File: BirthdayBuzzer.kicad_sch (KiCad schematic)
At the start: 14 parts, among them J3 Conn_ARM_SWD_TagConnect_TC203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, SW1 SW_Push, U1 PIC18F15Q41-I/SS

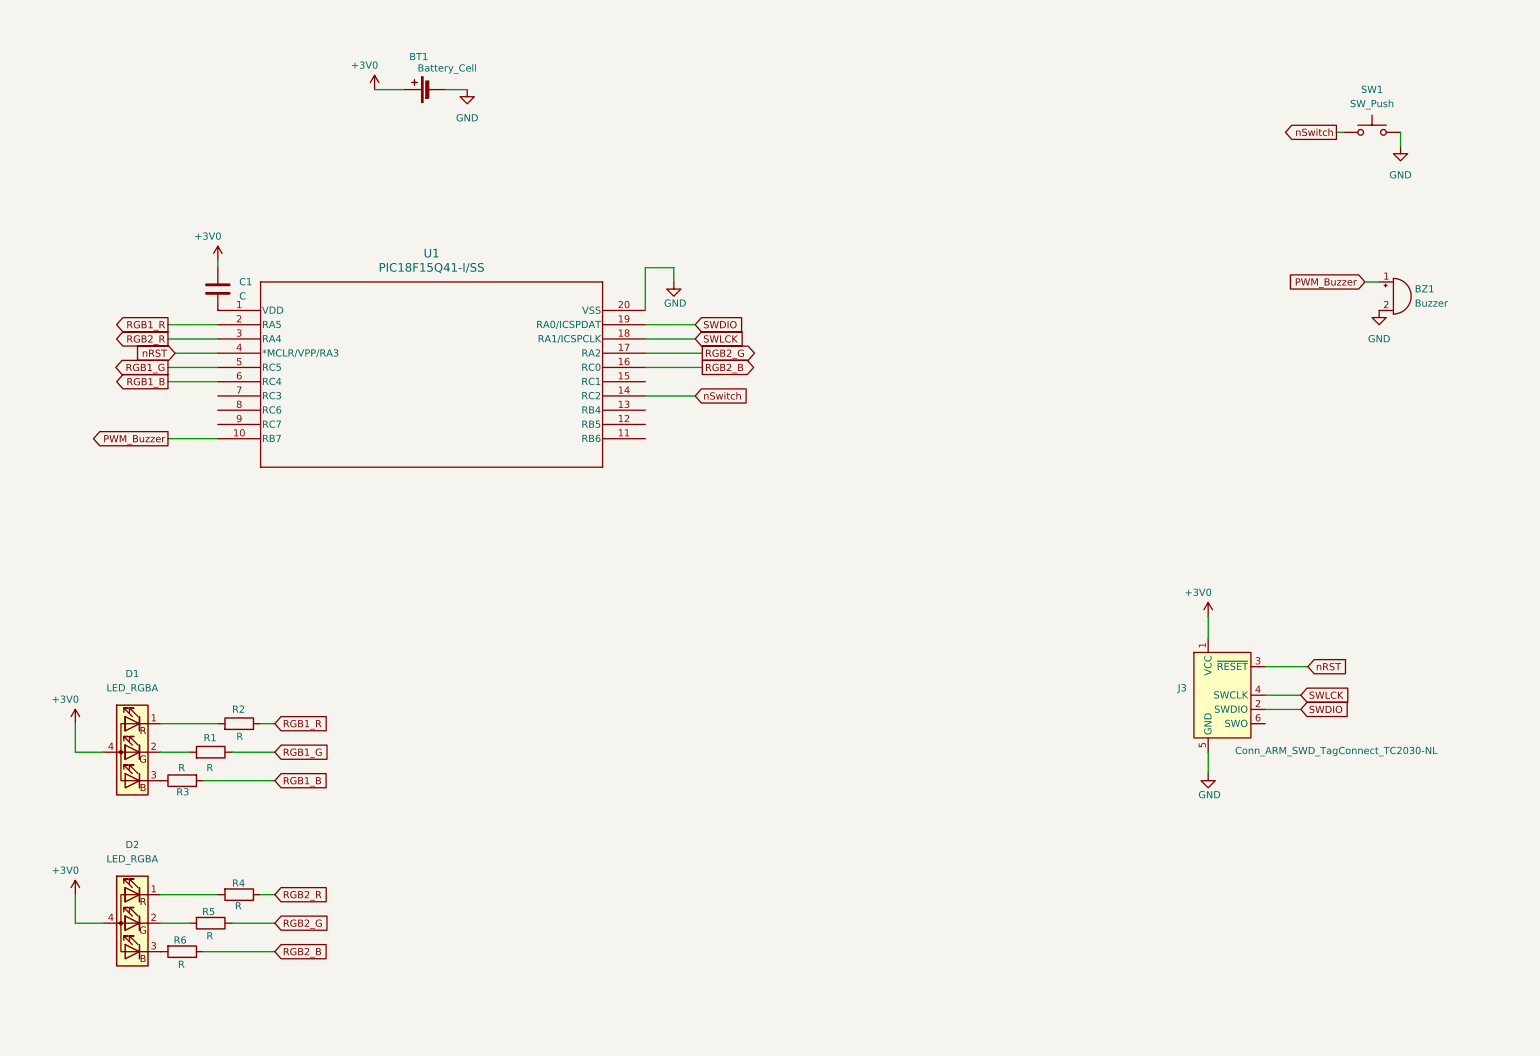
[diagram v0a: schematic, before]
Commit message: Cleaned up schematics and added notes
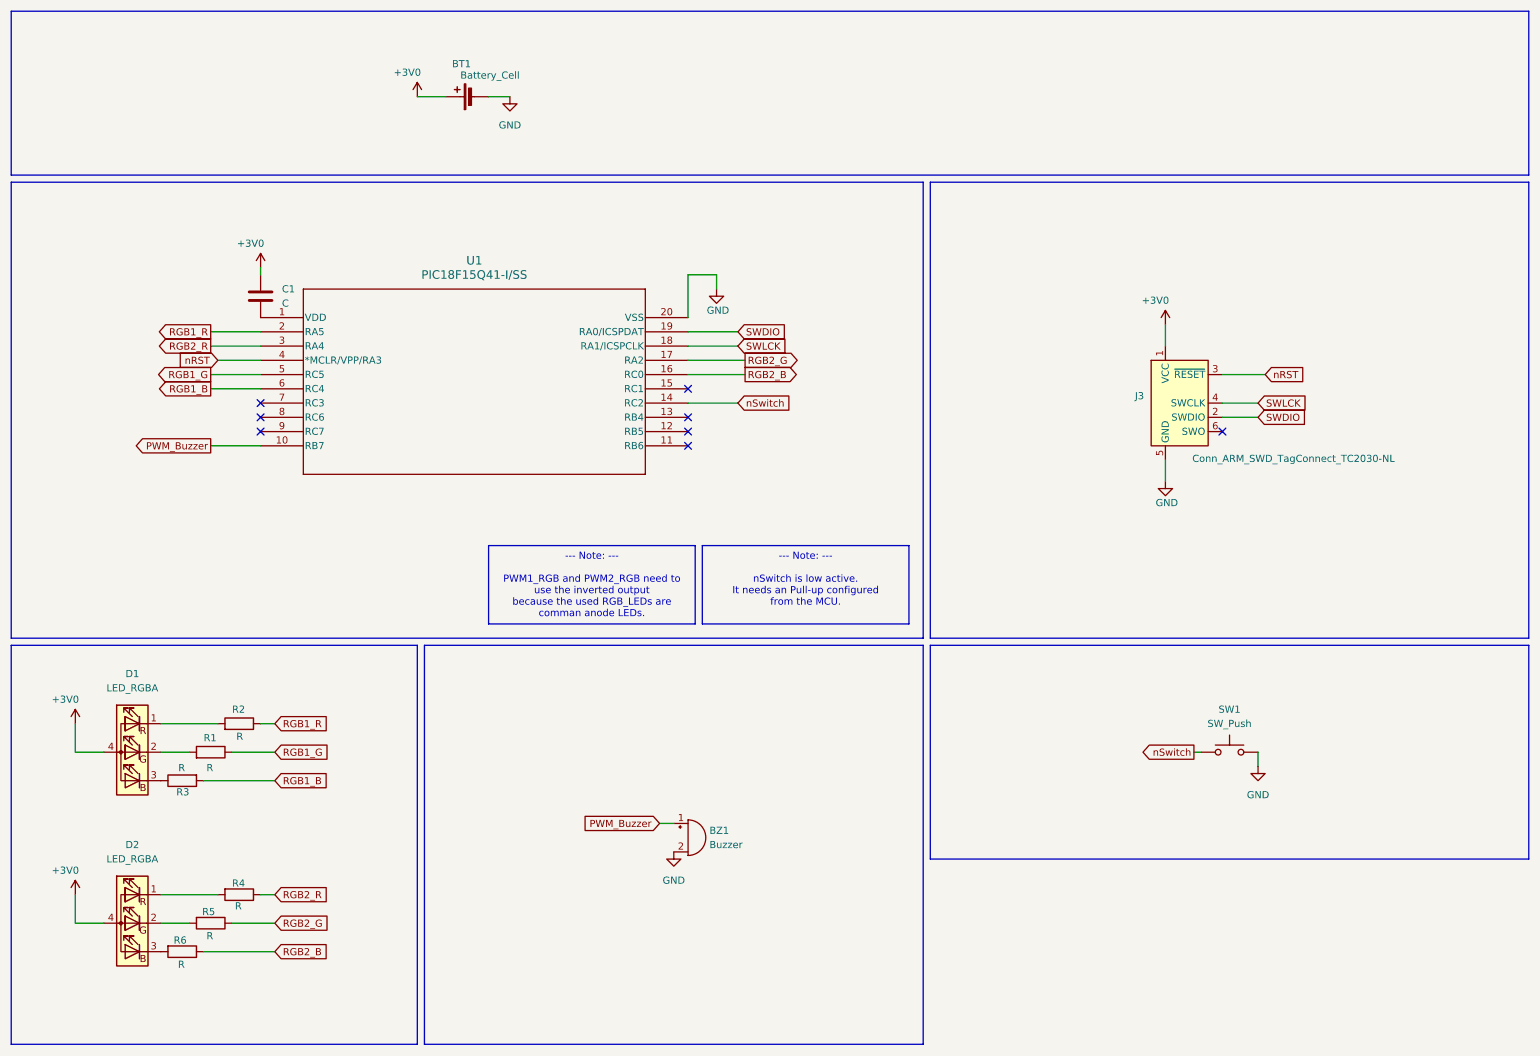
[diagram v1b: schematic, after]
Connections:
- no-connect marks 0 -> 8
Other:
- title: (none) -> BirthdayBuzzer
- moved on the sheet: BT1, BZ1, C1, J3, SW1, U1
